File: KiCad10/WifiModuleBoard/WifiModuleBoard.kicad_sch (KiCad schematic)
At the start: 11 parts, among them J2 Conn_01x07_Pin, J3 TC2030, J4 Conn_01x05_Pin, U1 ESP32-C5-WROOM-1U-N8R8

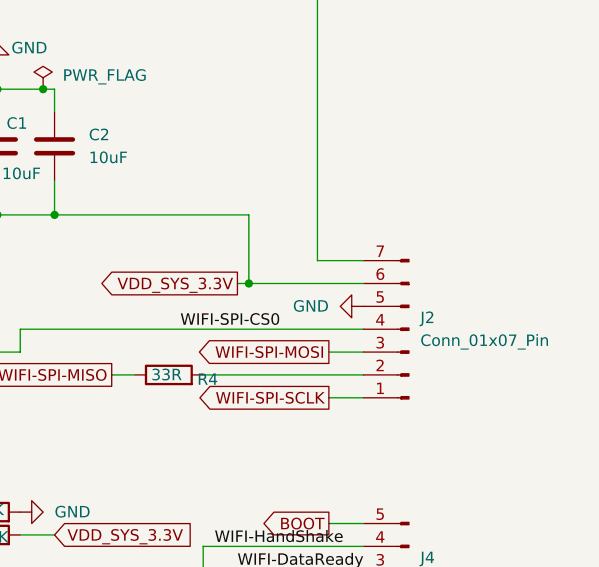
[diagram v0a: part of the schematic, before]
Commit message: etc
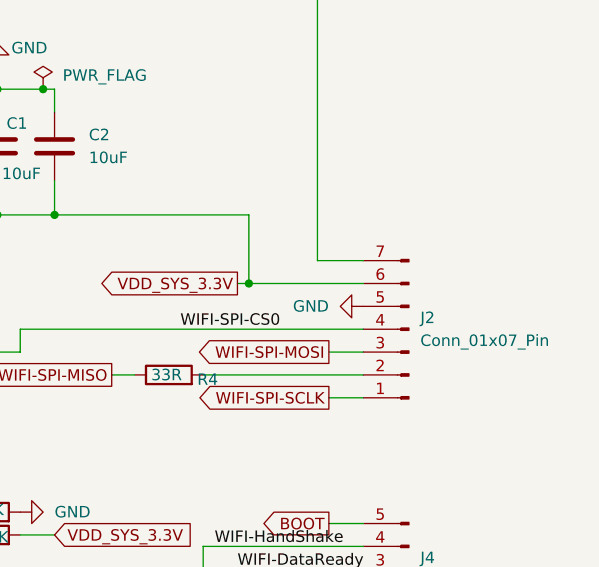
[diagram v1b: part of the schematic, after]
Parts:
- C1, C2, C3: Manufacturer Samsung Electro-Mechanics -> (none)
- R1, R2, R3: Manufacturer Uniroyal Elec -> (none)
- R4: LCSC Part# (none) -> C25105; MANUFACTURER (none) -> UNI-ROYAL; Manufacturer Uniroyal Elec -> (none); ManufacturerPartNumber (none) -> 0402WGF330JTCE
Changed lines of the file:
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@@
-			)
-		)
-		(property "Manufacturer" "Samsung Electro-Mechanics"
-			(at 115.57 66.04 0)
-			(hide yes)
-			(show_name no)
-			(do_not_autoplace no)
-			(effects
-				(font
-					(size 1.27 1.27)
-				)
 			)
 		)
@@
 		)
 		(property "LCSC Part#" "C15525"
-			(at 138.43 76.2 0)
-			(hide yes)
-			(show_name no)
-			(do_not_autoplace no)
-			(effects
-				(font
-					(size 1.27 1.27)
-				)
-			)
-		)
-		(property "Manufacturer" "Samsung Electro-Mechanics"
 			(at 138.43 76.2 0)
 			(hide yes)
@@
 			)
 		)
-		(property "Description" ""
+		(property "Description" "802.15.4, Bluetooth, WiFi 802.11b/g/n/ac/ax, Bluetooth v5.0, Thread, Zigbee® Transceiver Module 2.412GHz ~ 2.484GHz, 5.18GHz ~ 5.885GHz Antenna Not Included Surface Mount"
 			(at 110.49 106.68 0)
 			(hide yes)
@@
 		)
 		(property "LCSC Part#" ""
-			(at 110.49 106.68 0)
-			(hide yes)
-			(show_name no)
-			(do_not_autoplace no)
-			(effects
-				(font
-					(size 1.27 1.27)
-				)
-			)
-		)
-		(property "Manufacturer" ""
 			(at 110.49 106.68 0)
 			(hide yes)
@@
 			)
 		)
-		(property "Manufacturer" "Samsung Electro-Mechanics"
-			(at 144.78 76.2 0)
-			(hide yes)
-			(show_name no)
-			(do_not_autoplace no)
-			(effects
-				(font
-					(size 1.27 1.27)
-				)
-			)
-		)
 		(property "ManufacturerPartNumber" "CL05A106MQ5NUNC"
 			(at 144.78 76.2 0)
@@
 			)
 		)
-		(property "LCSC Part#" ""
+		(property "LCSC Part#" "C25105"
 			(at 157.48 101.6 90)
 			(hide yes)
@@
 			)
 		)
-		(property "Manufacturer" "Uniroyal Elec"
+		(property "ManufacturerPartNumber" "0402WGF330JTCE"
 			(at 157.48 101.6 90)
 			(hide yes)
@@
 			)
 		)
-		(property "ManufacturerPartNumber" ""
+		(property "MANUFACTURER" "UNI-ROYAL"
 			(at 157.48 101.6 90)
 			(hide yes)
@@
 		)
 		(property "LCSC Part#" "C25741"
-			(at 137.16 116.84 90)
-			(hide yes)
-			(show_name no)
-			(do_not_autoplace no)
-			(effects
-				(font
-					(size 1.27 1.27)
-				)
-			)
-		)
-		(property "Manufacturer" "Uniroyal Elec"
 			(at 137.16 116.84 90)
 			(hide yes)
@@
 			)
 		)
-		(property "Manufacturer" ""
-			(at 184.15 123.19 0)
-			(hide yes)
-			(show_name no)
-			(do_not_autoplace no)
-			(effects
-				(font
-					(size 1.27 1.27)
-				)
-			)
-		)
 		(property "ManufacturerPartNumber" ""
 			(at 184.15 123.19 0)
@@
 			)
 		)
-		(property "Manufacturer" ""
-			(at 184.15 96.52 0)
-			(hide yes)
-			(show_name no)
-			(do_not_autoplace no)
-			(effects
-				(font
-					(size 1.27 1.27)
-				)
-			)
-		)
 		(property "ManufacturerPartNumber" ""
 			(at 184.15 96.52 0)
@@
 		)
 		(property "LCSC Part#" "C25741"
-			(at 137.16 119.38 90)
-			(hide yes)
-			(show_name no)
-			(do_not_autoplace no)
-			(effects
-				(font
-					(size 1.27 1.27)
-				)
-			)
-		)
-		(property "Manufacturer" "Uniroyal Elec"
 			(at 137.16 119.38 90)
 			(hide yes)
@@
 			)
 		)
-		(property "Manufacturer" ""
-			(at 45.72 86.36 0)
-			(hide yes)
-			(show_name no)
-			(do_not_autoplace no)
-			(effects
-				(font
-					(size 1.27 1.27)
-				)
-			)
-		)
 		(property "ManufacturerPartNumber" ""
 			(at 45.72 86.36 0)
@@
 			(at 133.35 68.58 0)
 			(hide yes)
-			(show_name no)
-			(do_not_autoplace no)
-			(effects
-				(font
-					(size 1.27 1.27)
-				)
-			)
-		)
-		(property "Manufacturer" "Uniroyal Elec"
-			(at 133.35 68.58 0)
-			(hide yes)
